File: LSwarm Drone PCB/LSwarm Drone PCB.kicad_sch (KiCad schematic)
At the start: 116 parts, among them J2 Conn_01x06_Pin, J3 JST / BT2.0 Connector, J4 Conn_01x02_Pin, J5 Conn_01x02_Pin, J6 Conn_01x02_Pin, J7 Conn_01x02_Pin, J8 Conn_01x05_Pin, Q1 AO3400A, Q2 AO3400A, Q3 AO3400A, Q4 AO3400A, Q7 AO3407A, SW1 MSK12C02, SW2 SKRPACE010, SW3 SKRPACE010, U1 LSM6DSRTR, U12 AP2112K-3.3, U3 TPS61023DRLR, U4 SN74LVC1T45DBVR, U5 BMP581, U6 ESP32-C3-MINI-1U-N4, X1 X322512MSB4SI

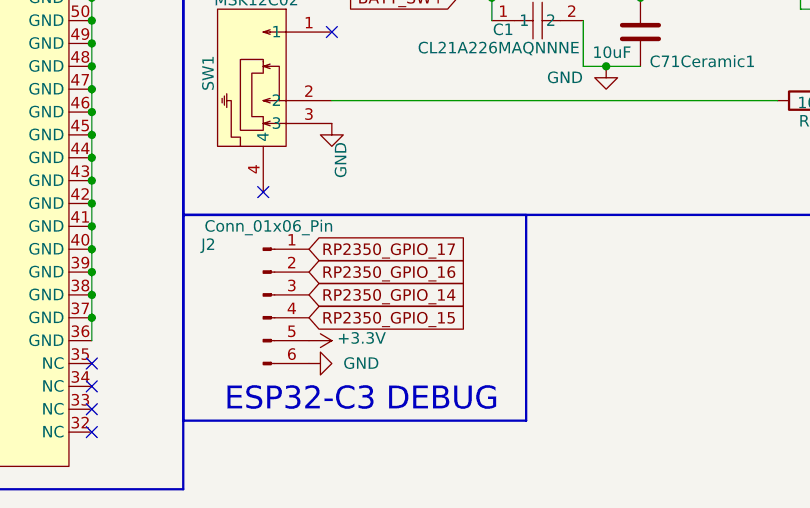
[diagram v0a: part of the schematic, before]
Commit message: sync
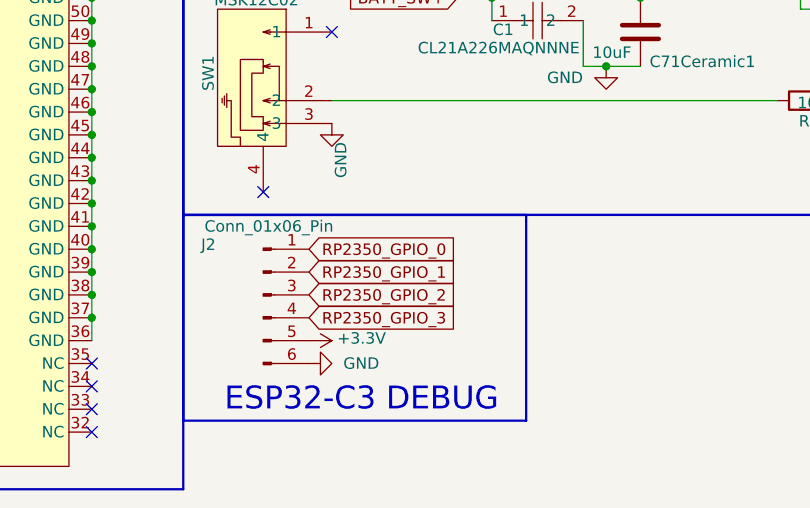
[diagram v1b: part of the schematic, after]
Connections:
- net RP2350_GPIO_14 is gone; now on net RP2350_GPIO_2: J2.3 (Pin_3)
- net RP2350_GPIO_15 is gone; now on net RP2350_GPIO_3: J2.4 (Pin_4)
- net RP2350_GPIO_16 is gone; now on net RP2350_GPIO_1: J2.2 (Pin_2)
- net RP2350_GPIO_17 is gone; now on net RP2350_GPIO_0: J2.1 (Pin_1)
